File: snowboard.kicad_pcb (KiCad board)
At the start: 4 copper layers, 80 x 46 mm, 30 parts, among them J1 Micro USB Port, J2 B2B-PH-K-S, Q1 S8050, Q2 S8050, SW1 BOOT, SW2 RESET, U1 ESP32-WROVER-E-N4R8, U2 CP2102N-A02-GQFN28R, U3 SPX3819M5-L-3-3, U4 MCP73831T-2ACI_OT

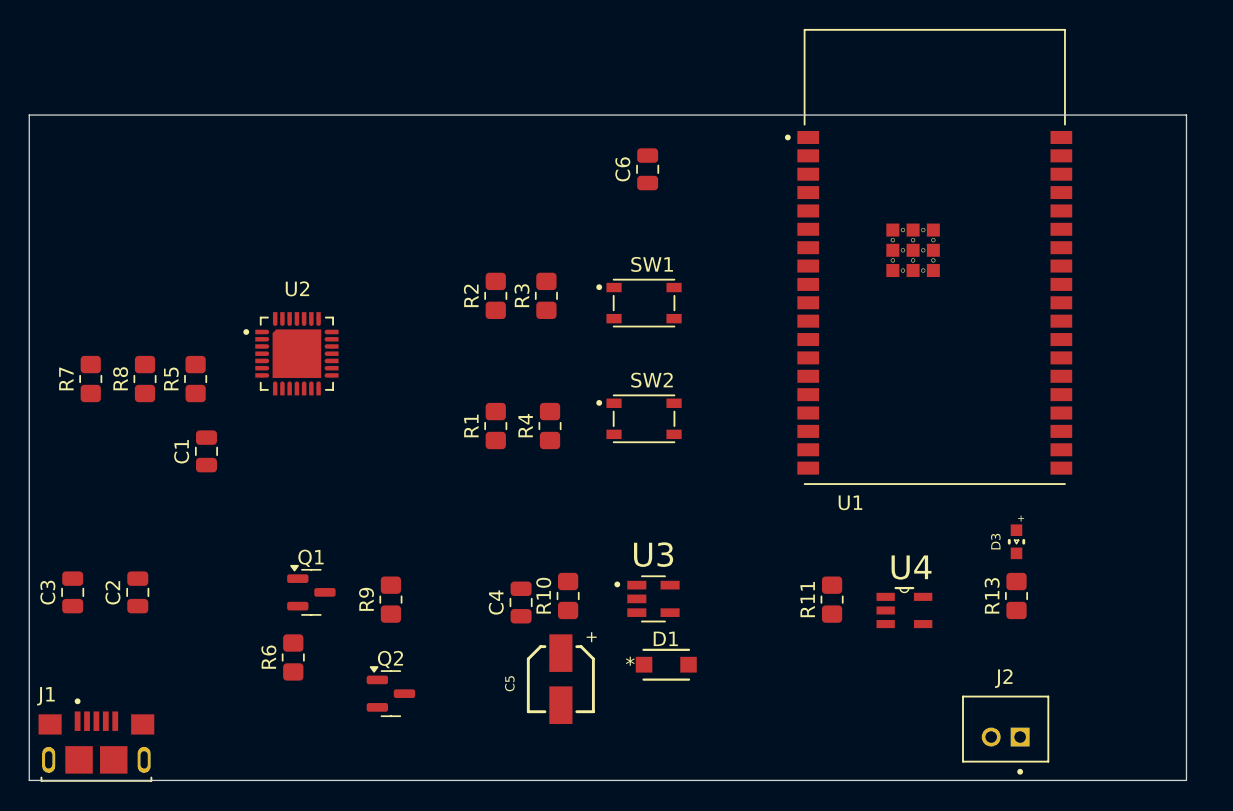
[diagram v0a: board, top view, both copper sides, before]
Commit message: PCB routing mostly done
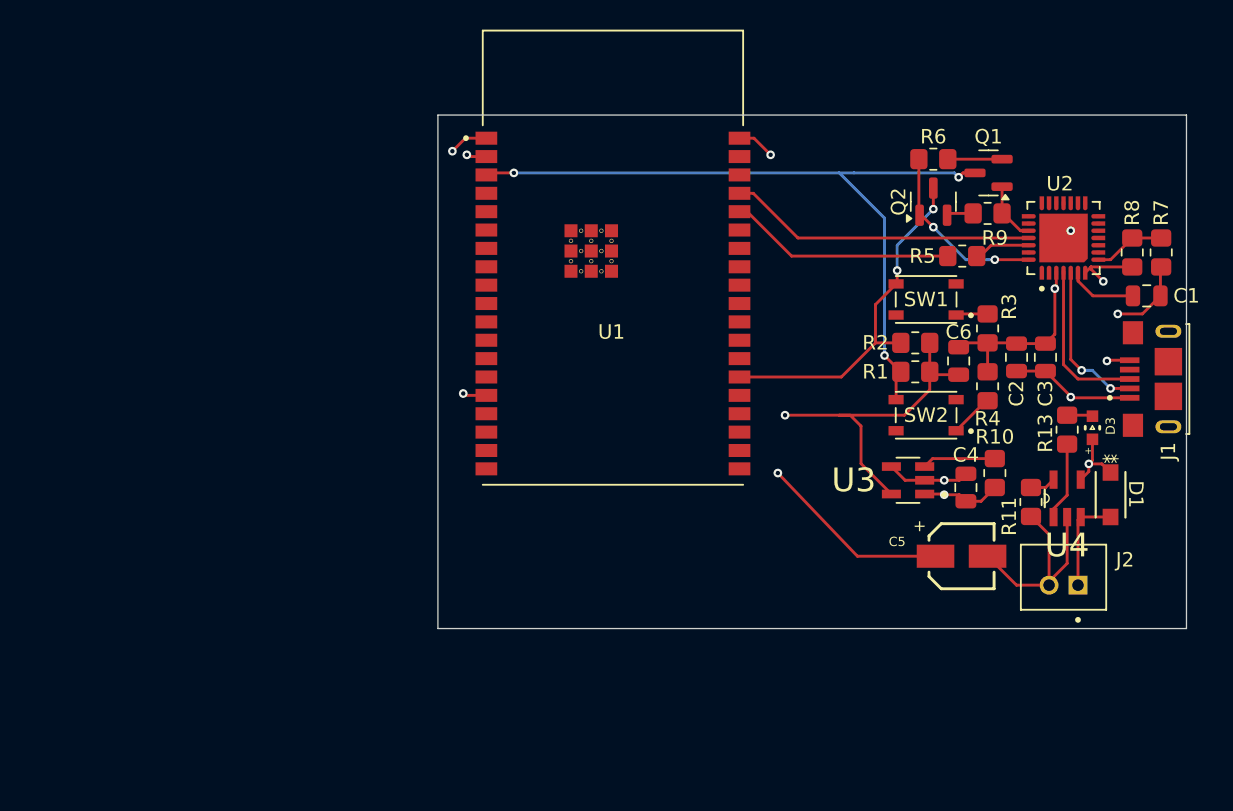
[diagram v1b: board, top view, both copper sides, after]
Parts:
- moved J1 78.6 mm to (184.2, 127.2), turned to 90 degrees
- moved R7 74.5 mm to (183.8, 118.5), turned to -90 degrees
- moved C3 69.2 mm to (175.8, 125.8)
- moved R8 68.8 mm to (181.8, 118.5)
- moved C1 65.9 mm to (182.8, 121.5), turned to 0 degrees
- moved C2 62.9 mm to (173.8, 125.8)
- moved R6 56.1 mm to (168.0, 112.0), turned to 0 degrees
- moved Q1 55.1 mm to (171.8, 113.0), turned to 180 degrees
- moved R5 53.7 mm to (170.0, 118.8), turned to 0 degrees
- moved U2 53.6 mm to (177.0, 117.5), turned to 90 degrees
- moved Q2 50.6 mm to (168.0, 115.0), turned to 90 degrees
- moved R9 49.1 mm to (171.8, 115.8), turned to 0 degrees
- moved D1 32.9 mm to (180.2, 135.2), turned to -90 degrees
- moved C4 31.8 mm to (170.2, 134.8)
- moved R10 30.7 mm to (172.2, 133.8)
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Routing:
- net /AEN: track 0.00 -> 51.7 mm, vias 0 -> 3
- net GND: track 0.00 -> 48.8 mm, vias 0 -> 8
- net +3.3V: track 0.00 -> 38.6 mm, vias 0 -> 3
- net /IO0: track 0.00 -> 24.6 mm, vias 0 -> 2
- net VBUS: track 0.00 -> 23.9 mm, vias 0 -> 4
- net /TX: track 0.00 -> 21.3 mm
- net /RX: track 0.00 -> 15.7 mm
- net /DTR: track 0.00 -> 12.7 mm, vias 0 -> 2
- net /D_P: track 0.00 -> 11.3 mm
- net /D_N: track 0.00 -> 11.0 mm, vias 0 -> 2
- net +BATT: track 0.00 -> 6.60 mm
- net Net-(U4-STAT): track 0.00 -> 5.43 mm
- net Net-(U3-EN): track 0.00 -> 5.08 mm
- net Net-(U2-VBUS): track 0.00 -> 4.97 mm
- net Net-(U2-VDD): track 0.00 -> 4.80 mm
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- added copper zone on In2.Cu, net +3.3V
- added copper zone on In1.Cu, net GND
- added copper zone on In2.Cu, net VBUS
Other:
- board size 80 x 46 mm -> 51.8 x 35.5 mm
